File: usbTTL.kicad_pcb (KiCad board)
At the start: 2 copper layers, 54.2 x 33.7 mm, 17 parts, among them J1 USB_A, J2 Conn_01x03_Pin, J3 Conn_01x03_Pin, J4 Conn_01x04_Pin, U1 CH340G, Y1 12Mhz

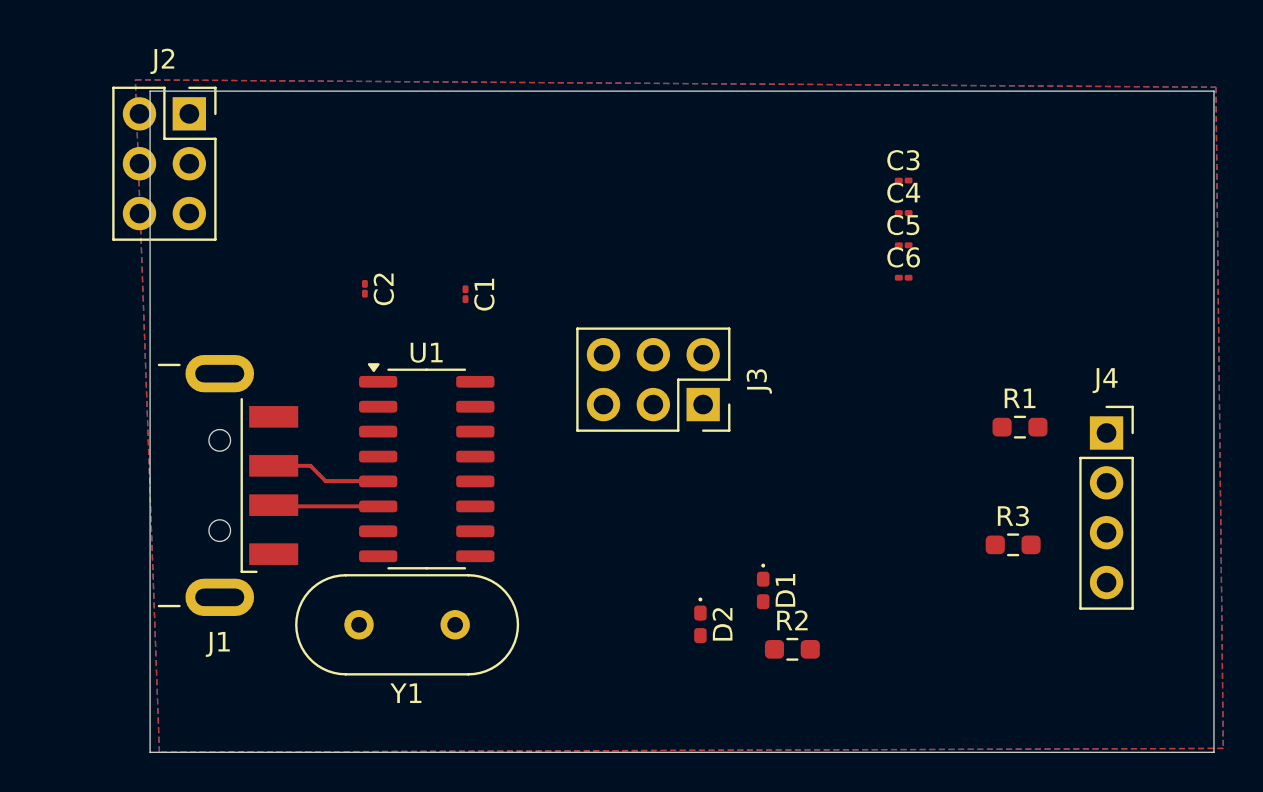
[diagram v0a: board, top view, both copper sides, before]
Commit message: sync 2
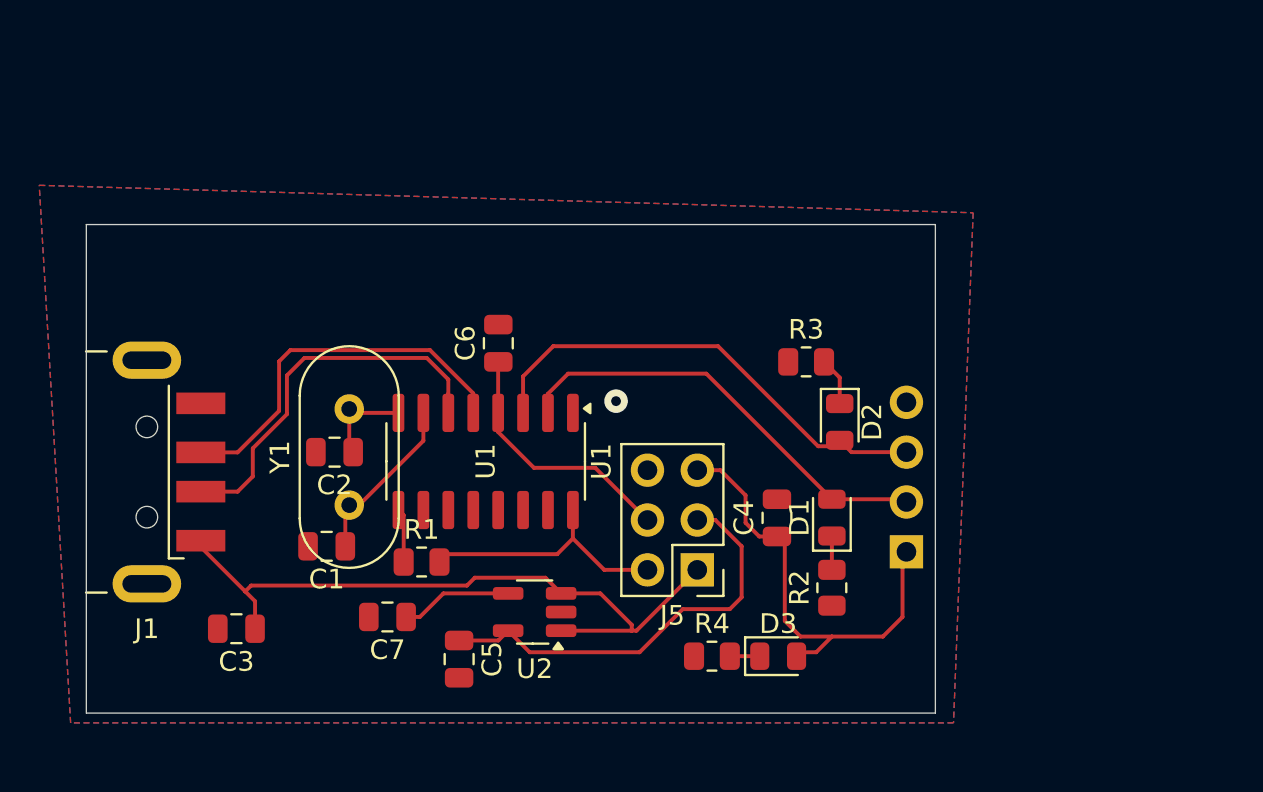
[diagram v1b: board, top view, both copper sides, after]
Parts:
- removed J2, J3: Conn_01x03_Pin, Connector_PinSocket_2.54mm:PinSocket_2x03_P2.54mm_Vertical
- added C7: 22pF, Capacitor_SMD:C_0805_2012Metric, F.Cu at (160.3, 125.4)
- added D3: PWR_LED, LED_SMD:LED_0805_2012Metric, F.Cu at (180.3, 127.4)
- added J5: Conn_01x06_Pin, Connector_PinHeader_2.54mm:PinHeader_2x03_P2.54mm_Vertical, F.Cu at (176.1, 123.0)
- added R4: 10k, Resistor_SMD:R_0805_2012Metric, F.Cu at (176.9, 127.4)
- added U2: SPX3819M5-L-3-3, Package_TO_SOT_SMD:SOT-23-5_HandSoldering, F.Cu at (167.8, 125.2)
- C1, C2, C3, C4, C6: footprint Capacitor_SMD:C_01005_0402Metric -> Capacitor_SMD:C_0805_2012Metric
- C5: value 10uF -> 0.01uF; footprint Capacitor_SMD:C_01005_0402Metric -> Capacitor_SMD:C_0805_2012Metric
- D1, D2: footprint LED_SMD:LED_0402_1005Metric_Pad0.77x0.64mm_HandSolder -> LED_SMD:LED_0805_2012Metric
- J4: footprint Connector_PinSocket_2.54mm:PinSocket_1x04_P2.54mm_Vertical -> Connector_PinHeader_2.54mm:PinHeader_1x04_P2.54mm_Horizontal; moved to B.Cu
- R1, R2, R3: footprint Resistor_SMD:R_0603_1608Metric_Pad0.98x0.95mm_HandSolder -> Resistor_SMD:R_0805_2012Metric
- moved C3 41.0 mm to (152.7, 126.0), turned to 180 degrees
- moved R1 31.3 mm to (162.1, 122.6)
- moved C5 31.0 mm to (164.0, 127.5), turned to -90 degrees
- moved C6 20.9 mm to (166.0, 111.5), turned to 90 degrees
- moved C4 16.8 mm to (180.2, 120.3), turned to 90 degrees
- moved C1 14.7 mm to (157.2, 121.8), turned to 180 degrees
- moved R3 14.1 mm to (181.7, 112.4)
- moved D2 12.5 mm to (183.4, 115.5)
- moved J4 11.9 mm to (186.8, 122.1)
- moved C2 8.47 mm to (157.7, 117.0), turned to 180 degrees
- moved Y1 8.15 mm to (158.4, 119.7), turned to 90 degrees
- moved D1 5.10 mm to (183.0, 120.3), turned to 90 degrees
- moved J1 3.78 mm to (141.2, 118.0)
- moved R2 3.73 mm to (183.0, 123.9), turned to 90 degrees
- moved U1 3.03 mm to (165.4, 117.5), turned to -90 degrees
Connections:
- D1 pad 1: /GND -> Net-(D1-K)
- D1 pad 2: Net-(D1-A) -> TX
- D2 pad 1: /GND -> Net-(D2-K)
- D2 pad 2: Net-(D2-A) -> RX
- R2 pad 1: Net-(D1-A) -> /GND
- R2 pad 2: TX -> Net-(D1-K)
- R3 pad 1: Net-(D2-A) -> /GND
- R3 pad 2: RX -> Net-(D2-K)
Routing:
- net /VCC: track 0.00 -> 36.5 mm
- net /5V: track 0.00 -> 35.1 mm
- net RX: track 0.00 -> 25.3 mm
- net TX: track 0.00 -> 22.2 mm
- net /3v3: track 0.00 -> 21.6 mm
- net USB_D-: track 5.35 -> 20.6 mm
- net USB_D+: track 5.65 -> 20.4 mm
- net /V3: track 0.00 -> 13.0 mm
- net Net-(U1-XI): track 0.00 -> 8.74 mm
- net Net-(U2-BP): track 0.00 -> 5.70 mm
- net Net-(U1-XO): track 0.00 -> 5.48 mm
- net Net-(U1-~{CTS}): track 0.00 -> 2.76 mm
- net Net-(D2-K): track 0.00 -> 2.46 mm
- net Net-(D1-K): track 0.00 -> 1.72 mm
- net Net-(D3-K): track 0.00 -> 1.52 mm
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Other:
- board size 54.2 x 33.7 mm -> 43.3 x 24.9 mm
